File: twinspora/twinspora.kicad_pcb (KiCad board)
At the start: 4 copper layers, 76.9 x 36.9 mm, 176 parts, among them J1 TYPE-C-31-M-12, J10 XY-SH1_0-4A61, J12 XY-SH1_0-5A61, J13 Conn_01x02, J14 Conn_01x03, J15 Conn_01x03, J2 XT30U-M, J3 XT60PW-M, J4 Conn_01x02, J5 XY-SH1_0-3A61, J6 XY-SH1_0-3A61, J7 Conn_01x02, J8 XY-SH1_0-6A51, J9 XY-SH1_0-6A51, Q1 AO3401A, SW2 TS1187A26020, SW3 TS1187A26020, U1 STM32G473RBTx, U10 SRV05-4A, U11 SRV05-4A, U12 SRV05-4A, U2 SRV05-4A, U3 SRV05-4A, U4 XC6206P332MR, U5 CA-IF1044VD-Q1, U6 DRV8316CRRGFR, U7 DRV8316CRRGFR, U8 MT6701QT, U9 MT6701QT, X1 X322512MSB4SI

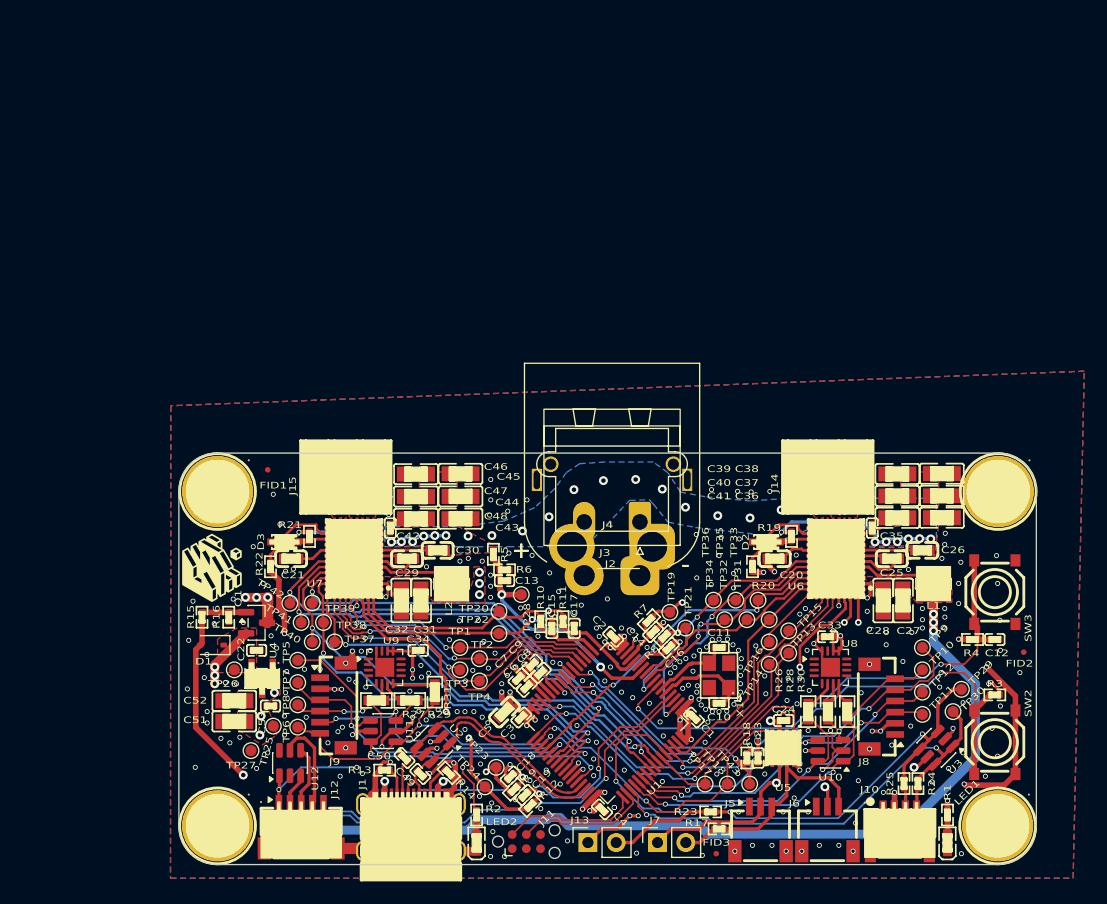
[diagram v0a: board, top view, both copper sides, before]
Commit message: NEW
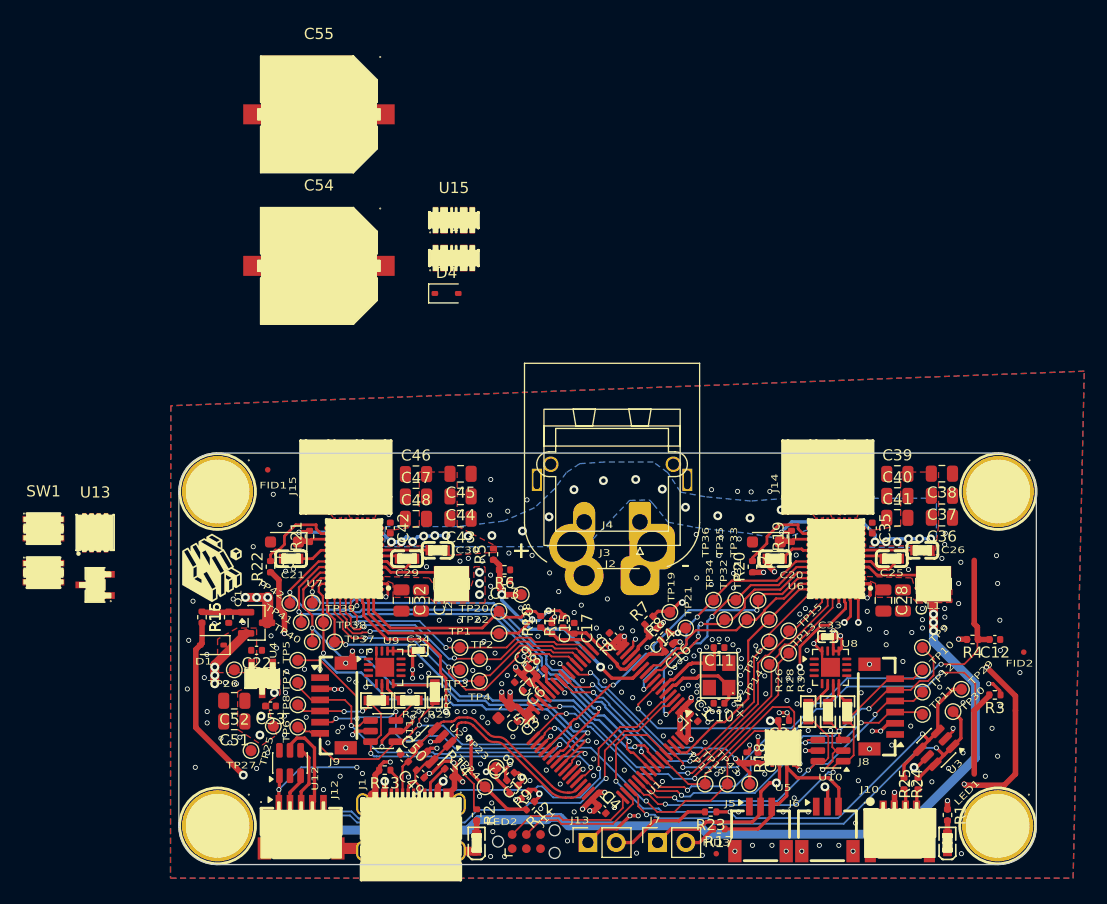
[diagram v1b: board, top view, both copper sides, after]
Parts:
- removed SW3: TS1187A26020, Switch:SW-SMD_4P-L5.2-W5.2-1
- added C54: EEEFT1H331GP, Capacitor_SMD_UWRL:CAP-SMD_BD10.0-L10.3-W10.3-LS11.0-R-RD, F.Cu at (89.1, 84.0)
- added C55: EEEFT1H331GP, Capacitor_SMD_UWRL:CAP-SMD_BD10.0-L10.3-W10.3-LS11.0-R-RD, F.Cu at (89.1, 70.4)
- added D4: 1N4148WS, Diode_SMD:D_SOD-323, F.Cu at (100.5, 86.5)
- added SW1: SKSGPAE010, Switch_UWRL:SW-SMD_SKSGAAE010, F.Cu at (64.4, 107.6)
- added U13: WSD4066DN, Transistor_FET_UWRL:DFN-8_L3.2-W3.1-P0.65-LS3.4-BL-EP, F.Cu at (69.0, 107.9)
- added U14: FMMT620TA, Transistor_BJT_UWRL:SOT-23-3_L2.9-W1.6-P1.90-LS2.8-BR, F.Cu at (69.0, 112.6)
- added U15: BK22C07-4DP/2-0_4V(800), Connector_HRS_BK22:CONN-SMD_4P-P0.40_BAM04-08073-0414, F.Cu at (101.2, 79.9)
- added U16: BK22C07-4DP/2-0_4V(800), Connector_HRS_BK22:CONN-SMD_4P-P0.40_BAM04-08073-0414, F.Cu at (101.2, 83.3)
- C1, C10, C11, C12, C13, C14, C15, C16, C17, C18, C19, C2, C22, C23, C24, C3, C35, C4, C42, C49, C50, C53, C6, C7, C8, C9: footprint Basic_Capacitors_Resistors:C0402 -> Capacitor_SMD:C_0402_1005Metric
- C27, C28, C31, C32, C36, C37, C38, C39, C40, C41, C43, C44, C45, C46, C47, C48, C51, C52: footprint Basic_Capacitors_Resistors:C0805 -> Capacitor_SMD:C_0805_2012Metric
- C5: footprint Basic_Capacitors_Resistors:C0603 -> Capacitor_SMD:C_0603_1608Metric
- D2, D3: value BZT52B5V1S -> BZT52B5V1S_C19077434; footprint Diode:SOD-323_L1.7-W1.3-LS2.6-RD -> Diode_SMD:D_SOD-323_HandSoldering
- R1, R10, R11, R12, R13, R14, R15, R16, R17, R18, R19, R2, R20, R21, R22, R23, R24, R25, R3, R4, R5, R6, R7, R8, R9: footprint Basic_Capacitors_Resistors:R0402 -> Resistor_SMD:R_0402_1005Metric
- SW2: value TS1187A26020 -> SKSGPAE010; footprint Switch:SW-SMD_4P-L5.2-W5.2-1 -> Switch_UWRL:SW-SMD_SKSGAAE010
- moved SW2 86.7 mm to (64.4, 111.5), turned to 0 degrees
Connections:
- C20 pad 2: Net-(U6-AVDD) -> Net-(U6-DRVOFF)
- C21 pad 2: Net-(U7-AVDD) -> Net-(U7-DRVOFF)
- C25 pad 1: Net-(U6-CPL) -> unconnected-(C25-Pad1)
- C25 pad 2: Net-(U6-CPH) -> unconnected-(C25-Pad2)
- C26 pad 2: Net-(U6-CP) -> unconnected-(C26-Pad2)
- C29 pad 1: Net-(U7-CPL) -> unconnected-(C29-Pad1)
- C29 pad 2: Net-(U7-CPH) -> unconnected-(C29-Pad2)
- C30 pad 2: Net-(U7-CP) -> unconnected-(C30-Pad2)
- L1 pad 2: Net-(U6-SW_BK) -> Net-(L1-Pad2)
- L2 pad 2: Net-(U7-SW_BK) -> Net-(L2-Pad2)
- R20 pad 2: Net-(U6-nFAULT) -> Net-(U6-nSLEEP)
- R22 pad 2: Net-(U7-nFAULT) -> Net-(U7-nSLEEP)
- SW2 pad 2: +3.3V -> /BOOT
- SW2 pad 3: /BOOT -> +3.3V
- U6 pad 13: /PHA1 -> /5V_BKOUT
- U6 pad 14: /PHA1 -> unconnected-(U6-OUTA-Pad14)
- U6 pad 16: /PHB1 -> unconnected-(U6-OUTB-Pad16)
- U6 pad 17: /PHB1 -> unconnected-(U6-OUTB-Pad17)
- U6 pad 19: /PHC1 -> Net-(L1-Pad2)
- U6 pad 20: /PHC1 -> GND
- U6 pad 21: unconnected-(U6-DRVOFF-Pad21) -> Net-(U6-DRVOFF)
- U6 pad 22: Net-(U6-nFAULT) -> Net-(D2-K)
- U6 pad 23: Net-(D2-K) -> Net-(U6-nSLEEP)
- U6 pad 25: Net-(U6-AVDD) -> unconnected-(U6-AVDD-Pad25)
- U6 pad 3: /5V_BKOUT -> /PHA1
- U6 pad 37: +3.3V -> unconnected-(U6-VREF/ILIM-Pad37)
- U6 pad 4: GND -> /PHA1
- U6 pad 5: Net-(U6-SW_BK) -> /PHB1
- U6 pad 6: Net-(U6-CPL) -> /PHB1
- U6 pad 7: Net-(U6-CPH) -> /PHC1
- U6 pad 8: Net-(U6-CP) -> /PHC1
- U7 pad 13: /PHA2 -> /BUCK
- U7 pad 14: /PHA2 -> unconnected-(U7-OUTA-Pad14)
- U7 pad 16: /PHB2 -> unconnected-(U7-OUTB-Pad16)
- U7 pad 17: /PHB2 -> unconnected-(U7-OUTB-Pad17)
- U7 pad 19: /PHC2 -> Net-(L2-Pad2)
- U7 pad 20: /PHC2 -> GND
- U7 pad 21: unconnected-(U7-DRVOFF-Pad21) -> Net-(U7-DRVOFF)
- U7 pad 22: Net-(U7-nFAULT) -> Net-(D3-K)
- U7 pad 23: Net-(D3-K) -> Net-(U7-nSLEEP)
- U7 pad 25: Net-(U7-AVDD) -> unconnected-(U7-AVDD-Pad25)
- U7 pad 3: /BUCK -> /PHA2
- U7 pad 37: +3.3V -> unconnected-(U7-VREF/ILIM-Pad37)
- U7 pad 4: GND -> /PHA2
- U7 pad 5: Net-(U7-SW_BK) -> /PHB2
- U7 pad 6: Net-(U7-CPL) -> /PHB2
- U7 pad 7: Net-(U7-CPH) -> /PHC2
- U7 pad 8: Net-(U7-CP) -> /PHC2
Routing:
- net (no net): track 2.02 -> 23.1 mm
- net /PHB1: track 0.00 -> 10.8 mm
- net /PHB2: track 0.00 -> 10.2 mm
- net Net-(U7-nFAULT): track 7.83 -> 0.00 mm
- net Net-(U6-nFAULT): track 7.58 -> 0.00 mm
- net Net-(U6-SW_BK): track 6.78 -> 0.00 mm
- net Net-(U7-SW_BK): track 6.58 -> 0.00 mm
- net /PHC1: track 0.00 -> 6.42 mm
- net /PHC2: track 0.00 -> 6.17 mm
- net Net-(U7-CP): track 4.42 -> 0.00 mm
- net Net-(U6-CP): track 4.42 -> 0.00 mm
- net Net-(U6-CPL): track 3.98 -> 0.00 mm
- net Net-(U7-CPL): track 3.59 -> 0.00 mm
- net Net-(U7-AVDD): track 2.86 -> 0.00 mm
- net Net-(U6-AVDD): track 2.82 -> 0.00 mm
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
